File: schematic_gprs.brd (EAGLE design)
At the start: 64.9 x 62 mm, 46 parts, among them J1 Jumper Alimentaciones, Q1 MOSFET-NCHANNEL2N7000, Q2 MOSFET-NCHANNEL2N7000, T1 BC547, X1 LTI-SASF54GT

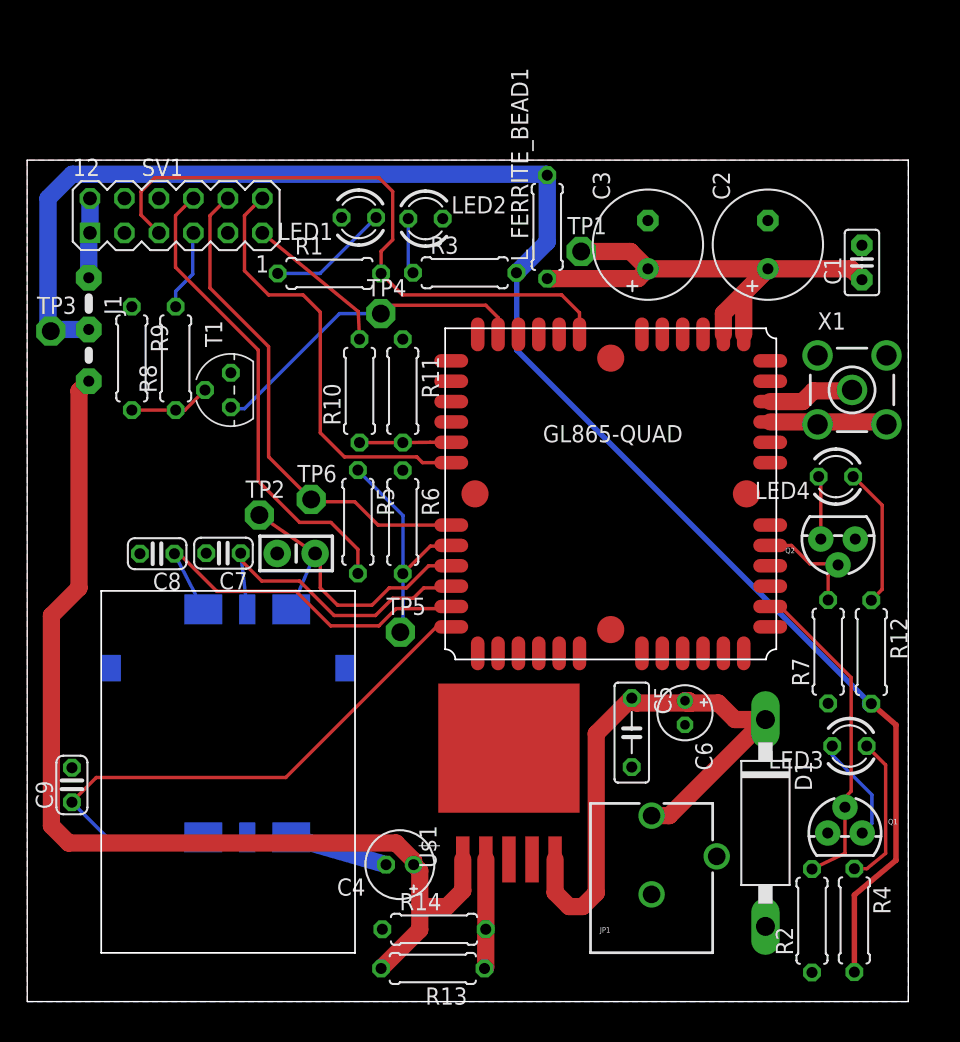
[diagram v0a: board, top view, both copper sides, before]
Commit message: Resultado Final
PCB  a espera de revisión por tutor el día 18/02/2015
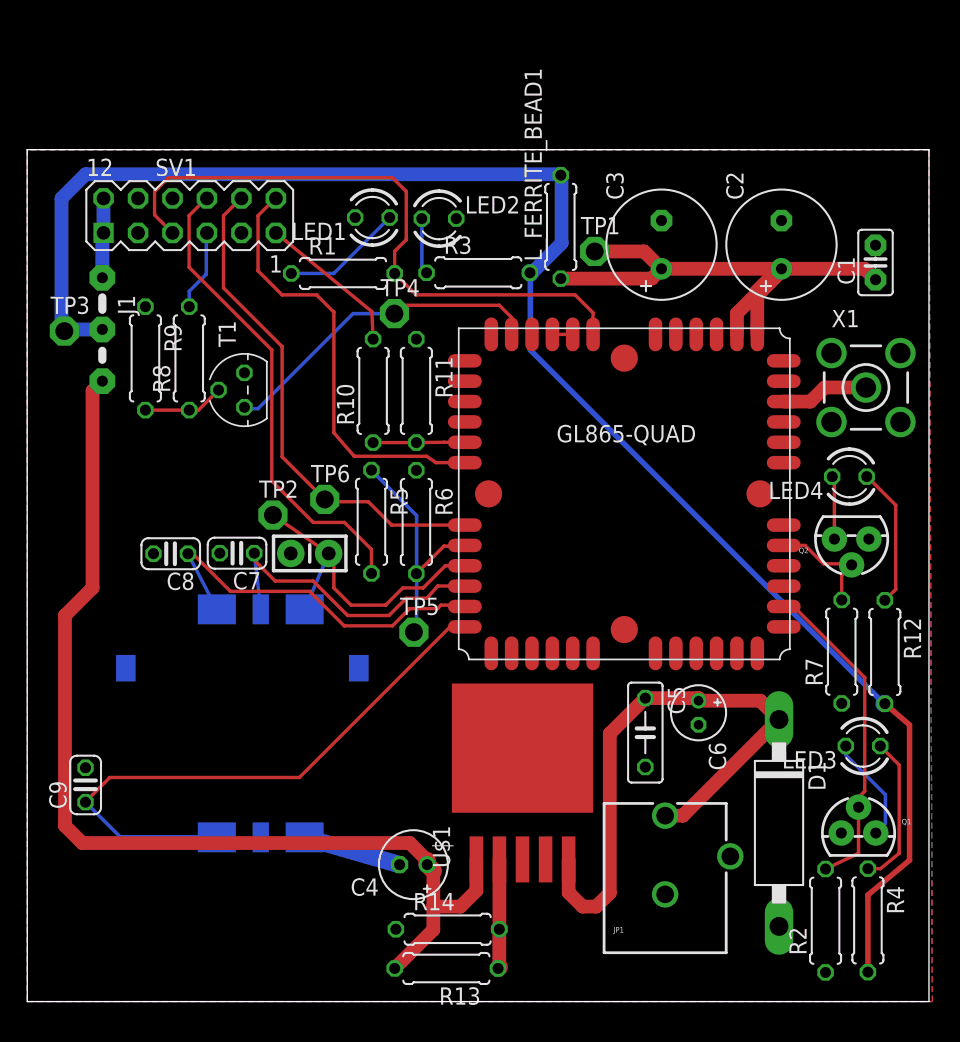
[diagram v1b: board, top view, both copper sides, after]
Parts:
- moved X1 1.04 mm to (61.8, 45.2)
- moved R9 1.00 mm to (8.70, 47.4)
- moved C1 1.00 mm to (62.5, 54.5)
- moved C10 1.00 mm to (20.8, 33.0)
- moved C2 1.00 mm to (55.6, 55.8)
- moved C3 1.00 mm to (46.7, 55.8)
- moved C4 1.00 mm to (28.4, 10.1)
- moved C5 1.00 mm to (45.5, 19.8)
- moved C6 1.00 mm to (49.5, 21.3)
- moved C7 1.00 mm to (15.5, 33.0)
- moved C8 1.00 mm to (10.6, 33.0)
- moved C9 1.00 mm to (4.29, 16.0)
- moved D1 1.00 mm to (55.4, 13.2)
- moved GSM/GPRS1 1.00 mm to (31.8, 25.2)
- moved J1 1.00 mm to (5.53, 51.4)
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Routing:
- net GND: track 15.9 -> 7.37 mm
- net N$17: track 0.00 -> 1.50 mm
- net N$11: track 44.4 -> 43.7 mm
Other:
- board size 64.9 x 62 mm -> 66.5 x 62.8 mm
